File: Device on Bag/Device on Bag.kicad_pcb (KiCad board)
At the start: 2 copper layers, 50.8 x 55.9 mm, 3 parts, among them J1 Screw_Terminal_01x02, U1 Adafruit-LSM6DSO32, U2 ESP32-DEVKIT-V1

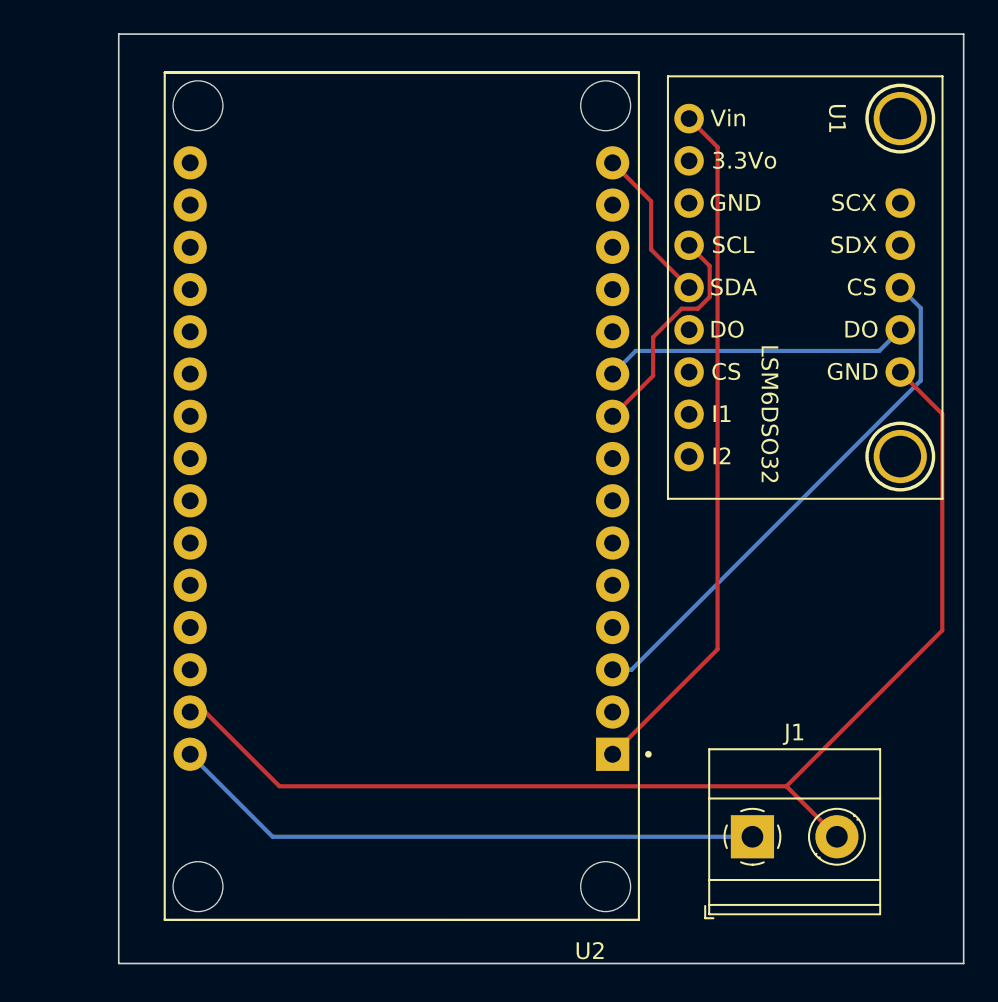
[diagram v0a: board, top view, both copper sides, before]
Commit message: update
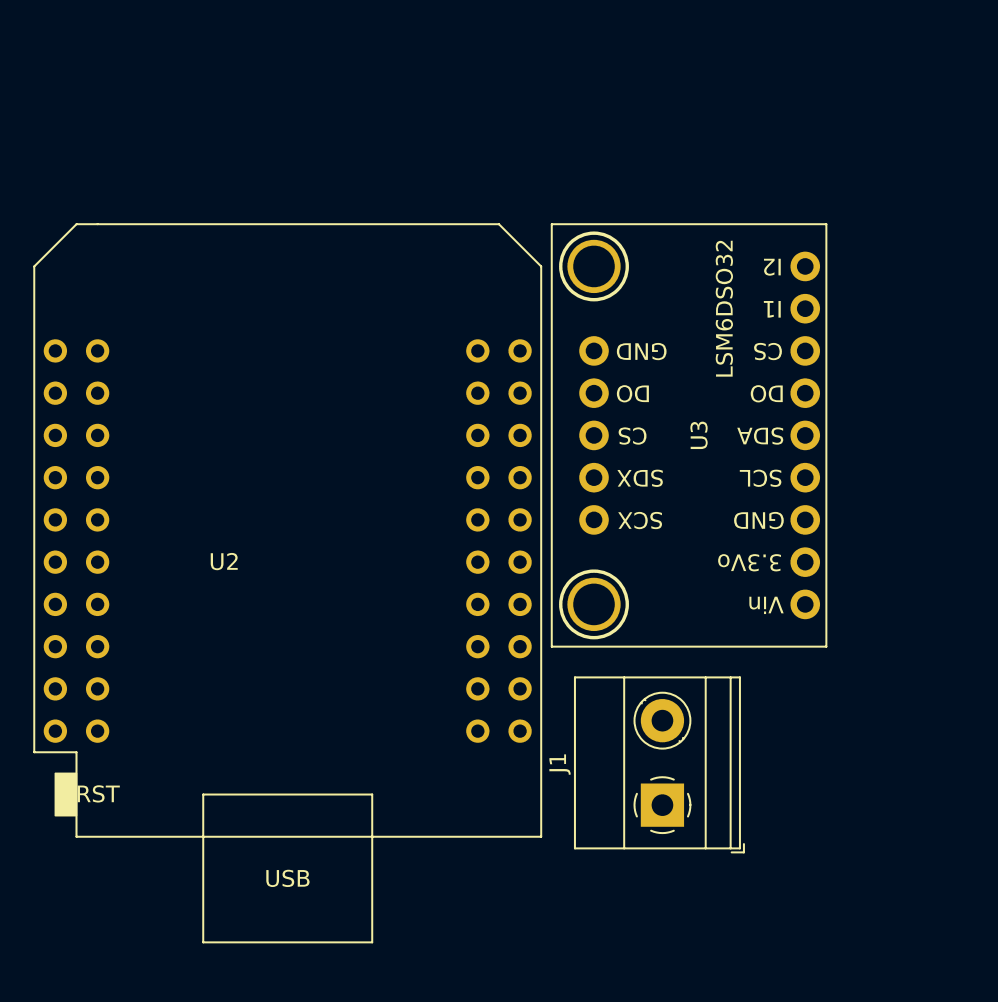
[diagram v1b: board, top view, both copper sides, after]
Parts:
- removed U1: Adafruit-LSM6DSO32, Adafruit-LSM6DSO32:Adafruit-LSM6DSO32
- added U3: Adafruit-LSM6DSO32, Adafruit-LSM6DSO32:Adafruit-LSM6DSO32, F.Cu at (154.3, 128.3)
- U2: value ESP32-DEVKIT-V1 -> mini_esp32; footprint ESP32-DEVKIT-V1:MODULE_ESP32_DEVKIT_V1 -> ESP32_mini_KiCad_Library:ESP32_mini
- moved U2 7.35 mm to (129.5, 134.6), turned to 0 degrees
- moved J1 5.73 mm to (152.1, 150.5), turned to 90 degrees
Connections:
- J1 pad 1: Net-(J1-Pad1) -> Vin
- U2 pad 1: 3.3v -> unconnected-(U2-Pad1)
- U2 pad 12: unconnected-(U2-Pad12) -> MOSI
- U2 pad 14: unconnected-(U2-Pad14) -> SS
- U2 pad 15: MOSI -> unconnected-(U2-Pad15)
- U2 pad 16: unconnected-(U2-Pad16) -> 3.3v
- U2 pad 29: GND -> unconnected-(U2-Pad29)
- U2 pad 3: SS -> unconnected-(U2-Pad3)
- U2 pad 30: Net-(J1-Pad1) -> unconnected-(U2-Pad30)
- U2 pad 8: unconnected-(U2-Pad8) -> SCK
- U2 pad 9: SCK -> unconnected-(U2-Pad9)
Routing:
- net GND: track 71.8 -> 0.00 mm
- net 3.3v: track 41.5 -> 0.00 mm
- net Net-(J1-Pad1): track 35.9 -> 0.00 mm
- net SS: track 31.8 -> 0.00 mm
- net MISO: track 18.4 -> 0.00 mm
- net SCK: track 13.8 -> 0.00 mm
- net MOSI: track 9.40 -> 0.00 mm
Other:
- board outline removed
